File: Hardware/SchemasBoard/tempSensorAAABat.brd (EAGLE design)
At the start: 22.2 x 24.1 mm, 9 parts, among them IC1 DS1820

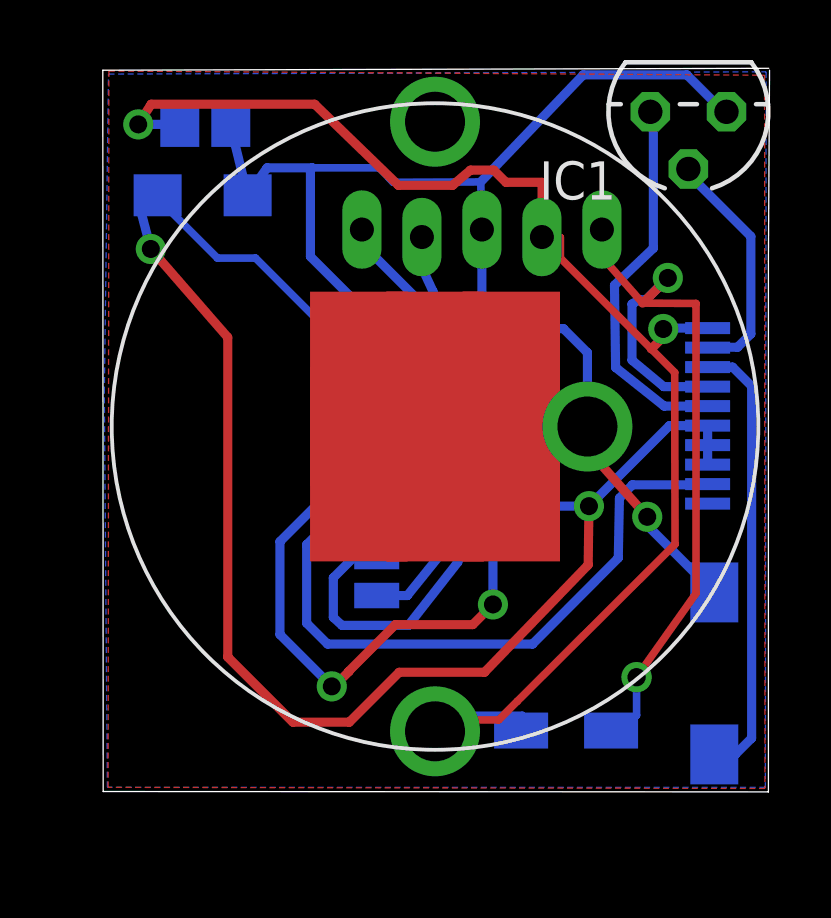
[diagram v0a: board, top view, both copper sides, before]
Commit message: aaa
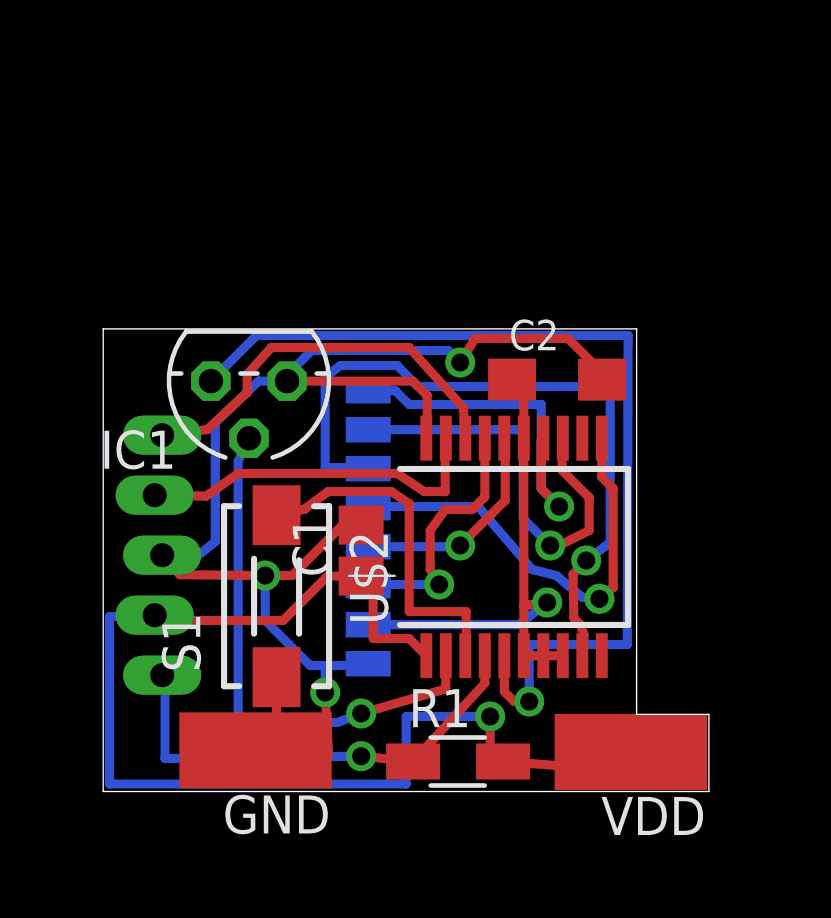
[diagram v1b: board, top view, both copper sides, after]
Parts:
- removed U$4: CR2032, rfm70:CR2032
- added GND, VDD: (no value), wirepad:SMD2,54-5,08
- moved U$1 30.4 mm to (23.1, 4.36), turned to 90 degrees
- moved IC1 17.2 mm to (4.86, 13.7)
- moved U$3 15.2 mm to (1.97, 7.88), turned to 90 degrees
- moved C1 15.1 mm to (8.60, 8.03), flipped to the top, turned to 90 degrees
- moved S1 14.8 mm to (5.78, 6.51), flipped to the top, turned to 90 degrees
- moved C2 13.3 mm to (15.1, 13.7), flipped to the top, turned to 0 degrees
- moved U$2 5.20 mm to (13.7, 8.15), flipped to the top, turned to 0 degrees
- moved R1 3.75 mm to (11.8, 1.00), flipped to the top
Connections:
- net N$5: now also VDD.1; no longer U$4.1
- net VD: now also GND.1; no longer U$4.3
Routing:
- net N$4: track 57.6 -> 17.9 mm, vias 2 -> 1
- net N$3: track 12.7 -> 32.2 mm, vias 0 -> 1
- net N$25: track 27.5 -> 15.5 mm, vias 2 -> 1
- net N$1: track 7.99 -> 18.4 mm, vias 0 -> 1
- net N$5: track 47.6 -> 40.5 mm, vias 2 -> 1
- net N$8: track 5.67 -> 11.9 mm
- net N$11: track 8.12 -> 13.5 mm
- net N$22: track 19.6 -> 14.7 mm, vias 2 -> 1
- net N$16: track 3.97 -> 8.58 mm, vias 0 -> 1
- net N$21: track 8.11 -> 12.2 mm, vias 0 -> 1
- net VD: track 45.7 -> 49.0 mm, vias 1 -> 3
- net N$2: track 14.9 -> 11.7 mm
- net N$20: track 4.25 -> 7.28 mm, vias 0 -> 1
- net N$12: track 12.7 -> 14.3 mm, vias 0 -> 1
- net N$23: track 22.3 -> 23.9 mm, vias 0 -> 1
- removed copper zone on layer 1, net VD
- removed copper zone on layer 16, net VDD
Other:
- board size 22.2 x 24.1 mm -> 20.2 x 15.4 mm

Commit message: aaa
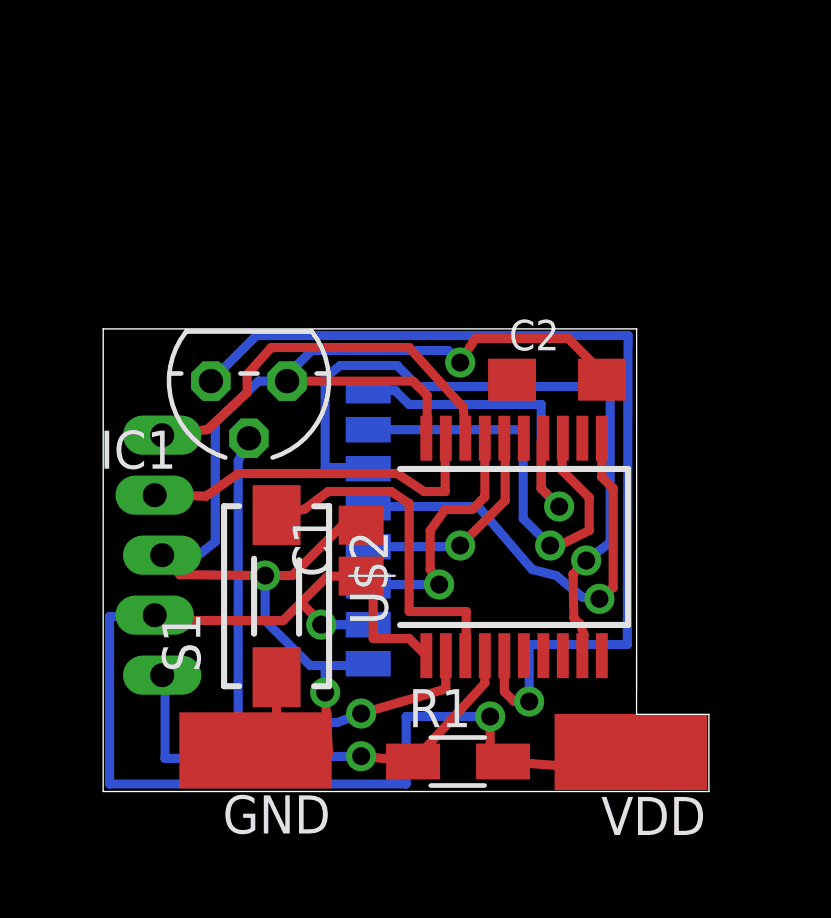
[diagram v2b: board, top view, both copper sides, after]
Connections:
- removed net N$4: C2.+, U$1.VDD, U$2.15, U$2.6, U$2.7, U$2.8
- removed net N$5: C1.1, R1.2, U$2.1, U$3.VDD, VDD.1
- new net N$7: C1.1, C2.+, R1.2, U$1.VDD, U$2.1, U$3.VDD, VDD.1
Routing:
- net N$7: track 0.00 -> 43.1 mm, vias 0 -> 2
- net N$5: track 40.5 -> 0.00 mm, vias 1 -> 0
- net N$4: track 17.9 -> 0.00 mm, vias 1 -> 0
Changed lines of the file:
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@@
 </signal>
 <signal name="N$23">
-<contactref element="U$2" pad="9"/>
 <contactref element="U$1" pad="MOSI"/>
-<wire x1="15.9717" y1="4.52704375" x2="15.999834375" y2="4.52704375" width="0.3048" layer="1"/>
 <wire x1="15.999834375" y1="4.52704375" x2="16.0256" y2="5.23665" width="0.3048" layer="1"/>
 <wire x1="16.0256" y1="5.23665" x2="15.89703125" y2="5.572" width="0.3048" layer="1"/>
@@
 <wire x1="7.4" y1="10.8" x2="8.7955625" y2="10.8" width="0.3048" layer="16"/>
 <wire x1="8.7955625" y1="10.8" x2="8.835025" y2="10.7605375" width="0.3048" layer="16"/>
+<contactref element="U$2" pad="9"/>
+<wire x1="15.999834375" y1="4.52704375" x2="15.9717" y2="4.52704375" width="0" layer="19" extent="1-1"/>
 </signal>
 <signal name="N$25">
@@
 <wire x1="12.1" y1="4.59874375" x2="12.0717" y2="4.52704375" width="0.3048" layer="1"/>
 </signal>
-<signal name="N$4">
-<contactref element="U$2" pad="6"/>
-<contactref element="U$2" pad="7"/>
+<signal name="N$7">
 <contactref element="U$1" pad="VDD"/>
 <contactref element="C2" pad="+"/>
-<contactref element="U$2" pad="8"/>
-<contactref element="U$2" pad="15"/>
-<wire x1="14.0217" y1="11.77704375" x2="14.0217" y2="13.1783" width="0.3048" layer="1"/>
-<wire x1="14.0217" y1="13.1783" x2="13.4" y2="13.8" width="0.3048" layer="1"/>
-<wire x1="14.0217" y1="11.77704375" x2="14.0217" y2="6.2" width="0.3048" layer="1"/>
-<wire x1="14.0217" y1="6.2" x2="14.0217" y2="4.52704375" width="0.3048" layer="1"/>
-<wire x1="14.0217" y1="4.52704375" x2="14.6717" y2="4.52704375" width="0.3048" layer="1"/>
-<wire x1="15.3217" y1="4.52704375" x2="15.3217" y2="4.5217" width="0.3048" layer="1"/>
-<wire x1="15.3217" y1="4.5217" x2="15.3" y2="4.5" width="0.3048" layer="1"/>
-<wire x1="14.6717" y1="4.52704375" x2="15.3217" y2="4.52704375" width="0.3048" layer="1"/>
-<wire x1="8.835025" y1="5.5605375" x2="13.8605375" y2="5.5605375" width="0.3048" layer="16"/>
-<wire x1="13.8605375" y1="5.5605375" x2="14.8" y2="6.3" width="0.3048" layer="16"/>
-<via x="14.8" y="6.3" extent="1-16" drill="0.6"/>
-<wire x1="14.8" y1="6.3" x2="14.0217" y2="6.2" width="0.3048" layer="1"/>
-<wire x1="13.4" y1="13.8" x2="13.63" y2="13.73" width="0" layer="19" extent="1-1"/>
-</signal>
-<signal name="N$5">
 <contactref element="R1" pad="2"/>
 <contactref element="U$3" pad="VDD"/>
@@
 <wire x1="10.19874375" y1="5.1" x2="10.7717" y2="4.52704375" width="0.3048" layer="1"/>
 <wire x1="8.6" y1="7.18" x2="7.48" y2="7.18" width="0.3048" layer="1"/>
-<wire x1="7.48" y1="7.18" x2="6" y2="5.7" width="0.3048" layer="1"/>
+<wire x1="7.48" y1="7.18" x2="6.595359375" y2="6.295359375" width="0.3048" layer="1"/>
+<wire x1="6.595359375" y1="6.295359375" x2="6" y2="5.7" width="0.3048" layer="1"/>
 <wire x1="6" y1="5.7" x2="1.88" y2="5.7" width="0.3048" layer="1"/>
 <wire x1="1.88" y1="5.7" x2="1.717253125" y2="5.877715625" width="0.3048" layer="1"/>
@@
 <wire x1="0.214425" y1="5.83603125" x2="1.18" y2="5.83603125" width="0.3048" layer="16"/>
 <wire x1="1.18" y1="5.83603125" x2="1.717253125" y2="5.877715625" width="0.3048" layer="16"/>
+<wire x1="8.835025" y1="5.5605375" x2="7.2685" y2="5.5605375" width="0.3048" layer="16"/>
+<wire x1="7.2685" y1="5.5605375" x2="7.2685" y2="5.562628125" width="0.3048" layer="16"/>
+<via x="7.2685" y="5.562628125" extent="1-16" drill="0.6"/>
+<wire x1="7.2685" y1="5.562628125" x2="7.2685" y2="5.62221875" width="0.3048" layer="1"/>
+<wire x1="7.2685" y1="5.62221875" x2="6.595359375" y2="6.295359375" width="0.3048" layer="1"/>
+<wire x1="9" y1="7.18" x2="13.63" y2="13.73" width="0" layer="19" extent="1-1"/>
 </signal>
 </signals>
